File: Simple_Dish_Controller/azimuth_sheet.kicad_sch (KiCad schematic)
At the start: 18 parts, among them J3 DE-15_VGA_FEMALE_CONN, J4 Conn_01x03_Pin, Q3 PZT2222A, Q4 PZT2222A, U2 74LS08, U3 74LS32, U5 NE555D

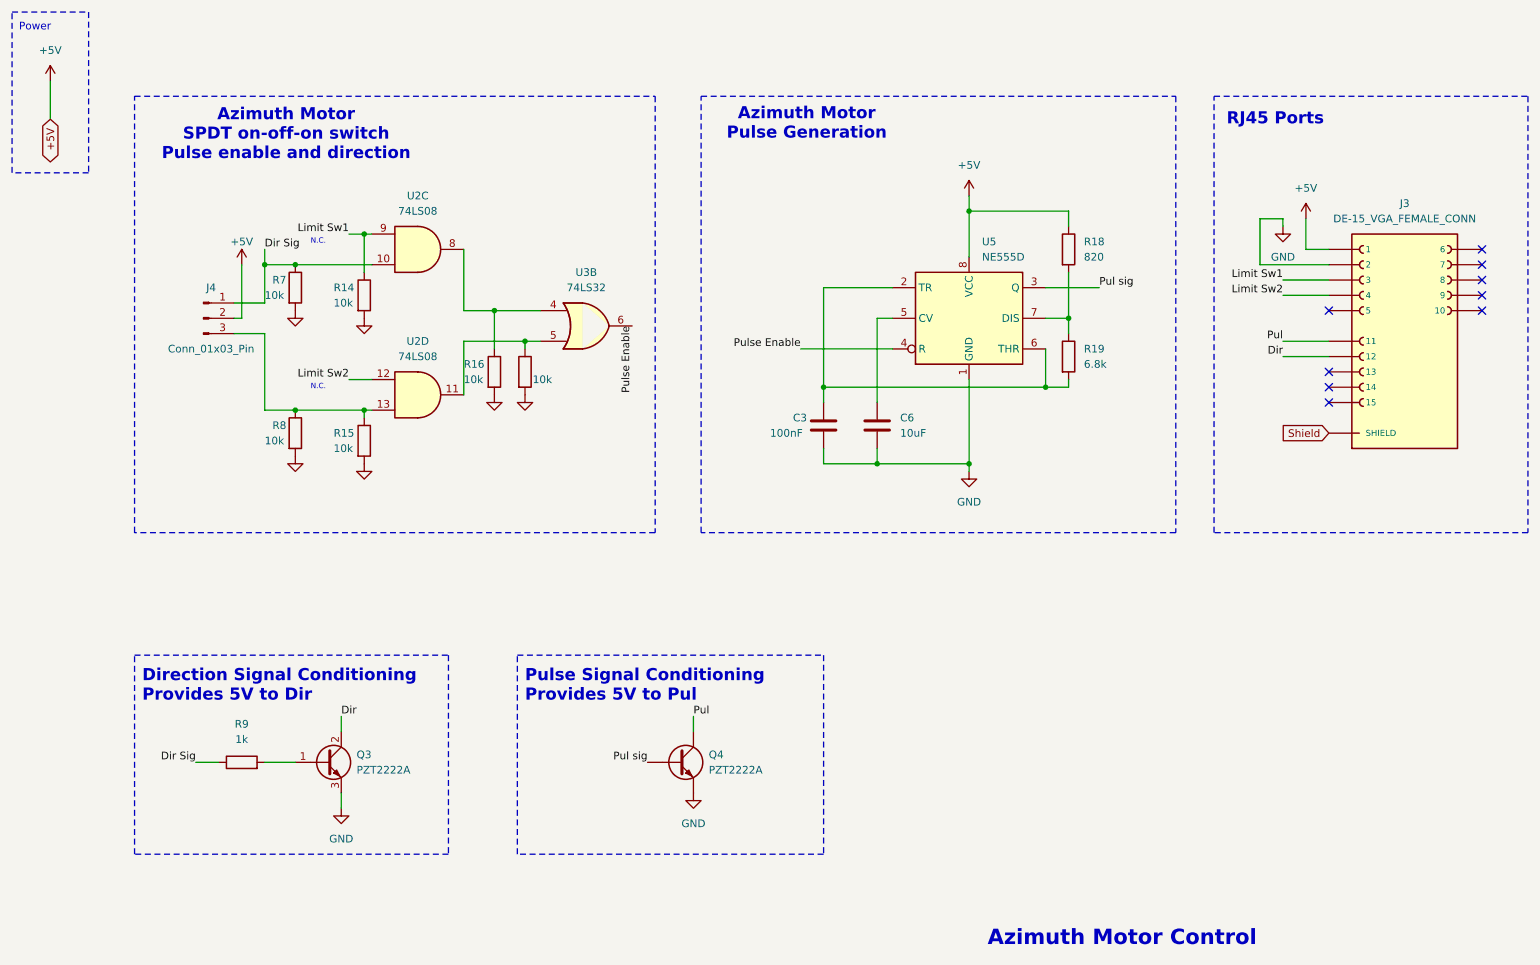
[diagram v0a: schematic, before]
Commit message: Updates
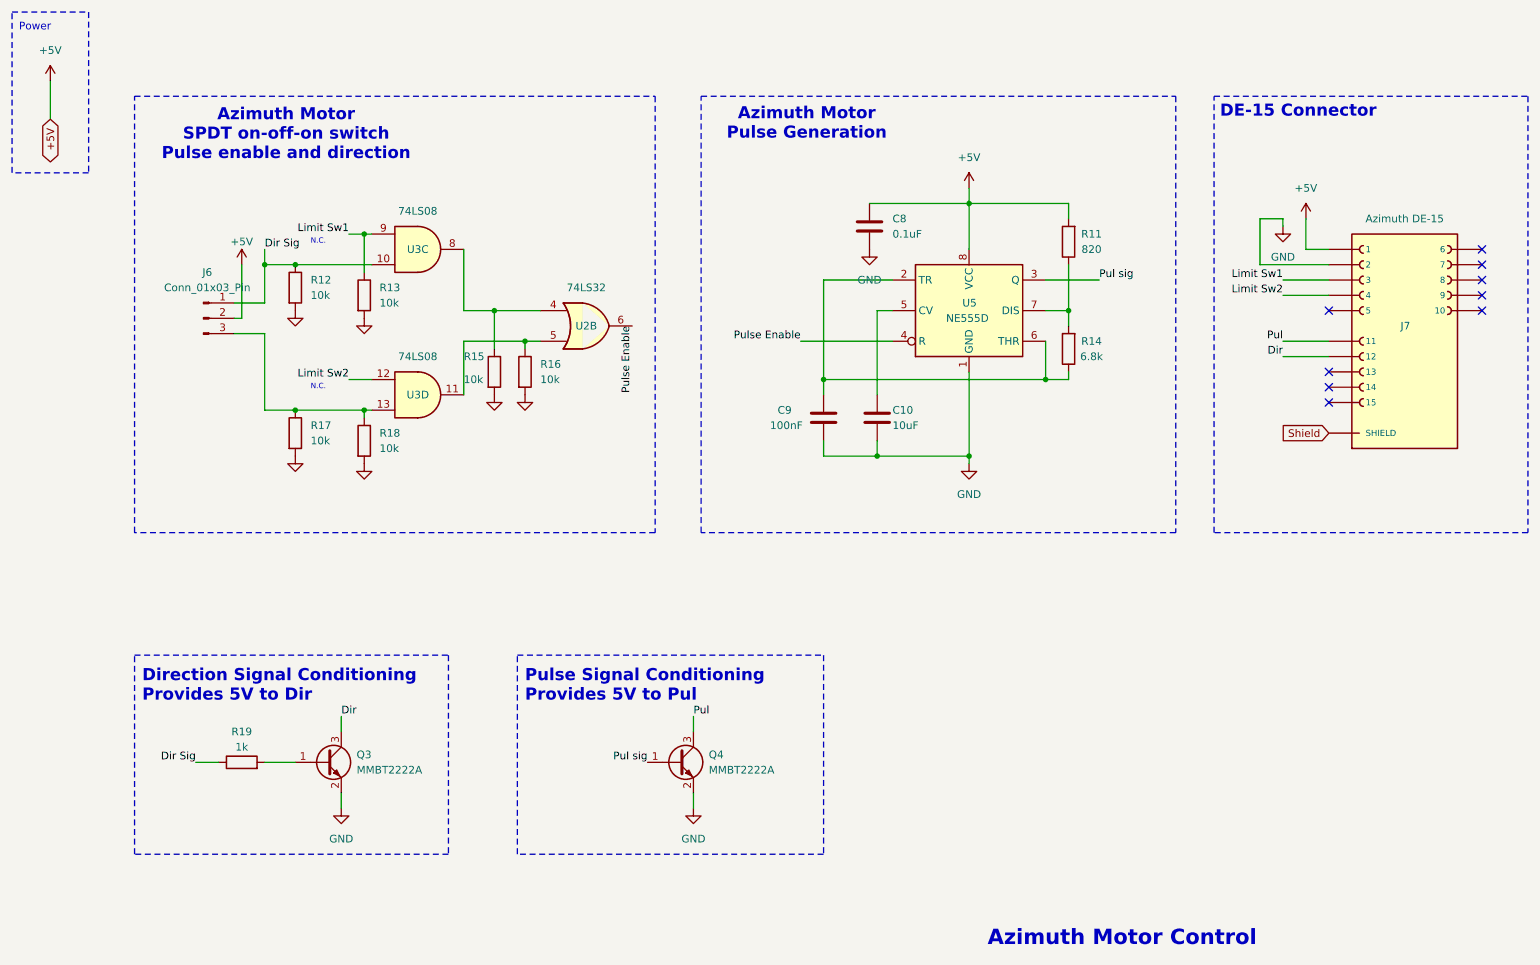
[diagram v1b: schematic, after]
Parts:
- removed C3: 100nF, DishFootprints:C_0805, symbol DishSymbols:CAP 100nF 0805
- removed C6: 10uF, DishFootprints:C_0805, symbol DishSymbols:CAP 10nF 0805
- removed J3: DE-15_VGA_FEMALE_CONN, DishFootprintsSupplier:DB15_VGA_FEMALE_CONN, symbol DishSymbolsSupplier:DE-15_VGA_FEMALE_CONN
- removed J4: Conn_01x03_Pin, DishFootprints:PinHeader_1x03_P2.54mm_Vertical, symbol DishSymbols:Conn_01x03_Pin
- removed Q3, Q4: PZT2222A, DishFootprints:SOT-223, symbol DishSymbols:PZT2222A
- removed R18: 820, DishFootprints:R_0805, symbol DishSymbols:RES 820 0805
- removed R19: 6.8k, DishFootprints:R_0805, symbol DishSymbols:RES 6.8k 0805
- removed R7, R8: 10k, Resistor_SMD:R_0805_2012Metric, symbol Device:R
- removed R9: 1k, Resistor_SMD:R_0805_2012Metric, symbol Device:R
- removed U2: 74LS08, DishFootprints:SOIC-14_3.9x8.7mm_P1.27mm, symbol DishSymbols:74LS08
- removed U3: 74LS32, DishFootprints:SOIC-14_3.9x8.7mm_P1.27mm, symbol DishSymbols:74LS32
- removed U5: NE555D, DishFootprints:SOIC-8_3.9x4.9mm_P1.27mm, symbol DishSymbols:NE555D
- added C10: 10uF, Capacitor_SMD:C_1206_3216Metric, symbol Device:C
- added C8: 0.1uF, Capacitor_SMD:C_1206_3216Metric, symbol Device:C
- added C9: 100nF, Capacitor_SMD:C_1206_3216Metric, symbol Device:C
- added J6: Conn_01x03_Pin, Connector_PinHeader_2.54mm:PinHeader_1x03_P2.54mm_Vertical, symbol Connector:Conn_01x03_Pin
- added J7: Azimuth DE-15, DishFootprints:DE15_VGA_FEMALE_CONN, symbol DishSymbols:DE-15_VGA_FEMALE_CONN
- added Q3, Q4: MMBT2222A, Package_TO_SOT_SMD:SOT-23, symbol Transistor_BJT:MMBT2222A
- added R11: 820, Resistor_SMD:R_1206_3216Metric, symbol Device:R
- added R12, R13, R18: 10k, Resistor_SMD:R_1206_3216Metric, symbol Device:R
- added R19: 1k, Resistor_SMD:R_1206_3216Metric, symbol Device:R
- added U2: 74LS32, Package_SO:SOIC-14_3.9x8.7mm_P1.27mm, symbol 74xx:74LS32
- added U3: 74LS08, Package_SO:SOIC-14_3.9x8.7mm_P1.27mm, symbol 74xx:74LS08
- added U5: NE555D, Package_SO:SOIC-8_3.9x4.9mm_P1.27mm, symbol Timer:NE555D
- R14: value 10k -> 6.8k; footprint Resistor_SMD:R_0805_2012Metric -> Resistor_SMD:R_1206_3216Metric
- R15, R16, R17: footprint Resistor_SMD:R_0805_2012Metric -> Resistor_SMD:R_1206_3216Metric
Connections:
- net +5V: now also C8.1, J6.2 (Pin_2), J7.1, R11.2, U5.8 (VCC)
- net Dir: now also J7.12, Q3.3 (C)
- net Dir Sig: now also J6.1 (Pin_1), R12.1, R19.1, U3.10
- net GND: now also C10.2, C8.2, C9.2, J7.2, Q3.2 (E), Q4.2 (E), R12.2, R13.2, R18.2, U5.1 (GND); no longer R14.2
- net Limit Sw1: now also J7.3, R13.1, U3.9; no longer R14.1
- net Limit Sw2: now also J7.4, U3.12
- net Pul: now also J7.11, Q4.3 (C)
- net Pul sig: now also Q4.1 (B), U5.3 (Q)
- net Pulse Enable: now also U2.6, U5.4 (R)
- net Shield: now also J7.SH1 (SHIELD), J7.SH2 (SHIELD)
- net at R15.1: now also U2.4, U3.8
- net at R17.1: now also J6.3 (Pin_3), R18.1, U3.13
- net at R16.1: now also U2.5, U3.11
- new net: Q3.1 (B), R19.2
- new net: C9.1, R14.1, U5.2 (TR), U5.6 (THR)
- new net: R11.1, R14.2, U5.7 (DIS)
- new net: C10.1, U5.5 (CV)
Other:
- note added: "DE-15 Connector"
- note removed: "RJ45 Ports"
